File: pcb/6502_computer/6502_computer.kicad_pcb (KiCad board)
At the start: 2 copper layers, 116.8 x 73.7 mm, 50 parts, among them J1 Conn_02x04_Odd_Even, J2 USB_B, J3 Conn_02x20_Odd_Even, J4 Conn_01x04, J5 Conn_01x02, J6 Conn_01x05, J8 Conn_01x05, Q1 NPN, SW1 SW_Push, SW2 SW_Push, SW3 SW_Push, U1 6502, U10 CH340N, U11 MC6840, U2 6551, U3 74LS139, U4 74LS138, U5 CY62256-70PC, U6 27C64, U7 74LS00, U8 DS1813-5+, U9 74LS93, X1 ACO-xxxMHz, Y1 1.8432MHz

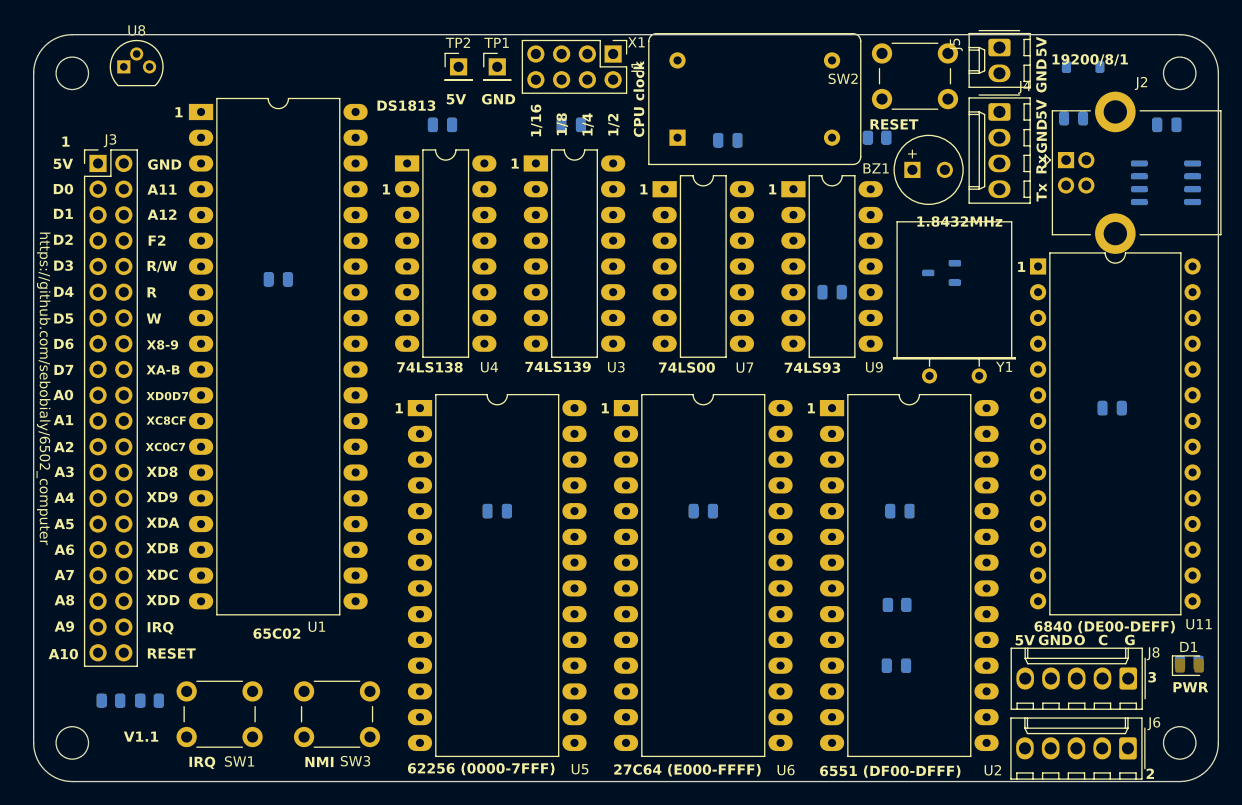
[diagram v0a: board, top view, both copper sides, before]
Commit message: routed 1.2 version
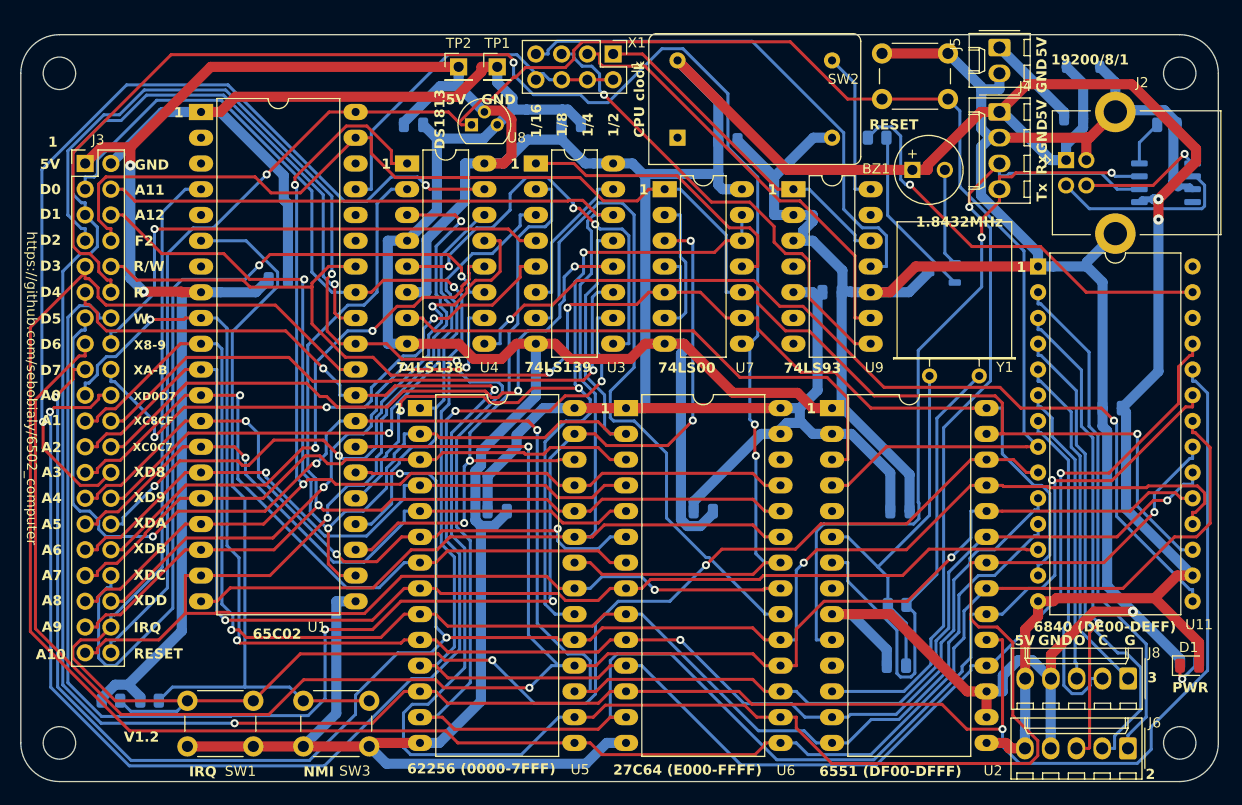
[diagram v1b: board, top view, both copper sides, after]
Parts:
- moved U8 34.8 mm to (108.0, 45.7)
- moved C6 2.86 mm to (102.2, 45.7)
- moved J3 1.27 mm to (69.8, 49.5)
- moved H2 1.27 mm to (67.3, 106.7)
- moved H4 1.27 mm to (67.3, 40.6)
- moved SW1 0.93 mm to (86.4, 107.0)
- moved SW3 0.93 mm to (97.9, 107.0)
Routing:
- net GND: track 0.00 -> 562.6 mm, vias 0 -> 1
- net VCC: track 0.00 -> 484.4 mm, vias 0 -> 4
- net /D1: track 0.00 -> 268.0 mm, vias 0 -> 3
- net /D2: track 0.00 -> 229.0 mm, vias 0 -> 3
- net /D3: track 0.00 -> 215.6 mm
- net /D4: track 0.00 -> 207.3 mm, vias 0 -> 3
- net /D0: track 0.00 -> 204.8 mm, vias 0 -> 2
- net /D6: track 0.00 -> 202.6 mm, vias 0 -> 3
- net /D7: track 0.00 -> 195.3 mm, vias 0 -> 4
- net /RES: track 0.00 -> 192.4 mm, vias 0 -> 1
- net /D5: track 0.00 -> 180.6 mm, vias 0 -> 4
- net /IRQ: track 0.00 -> 176.6 mm, vias 0 -> 2
- net /R: track 0.00 -> 163.5 mm, vias 0 -> 3
- net /W: track 0.00 -> 150.6 mm, vias 0 -> 4
- net /A11: track 0.00 -> 148.3 mm
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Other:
- board size 116.8 x 73.7 mm -> 118.1 x 73.7 mm
- board text added: "V1.2"
- board text removed: "V1.1"
